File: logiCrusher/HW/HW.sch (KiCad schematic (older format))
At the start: 11 parts, among them J1 Left, J3 Conn_02x05_Odd_Even, J4 Right, U3 R-783.3-0.5

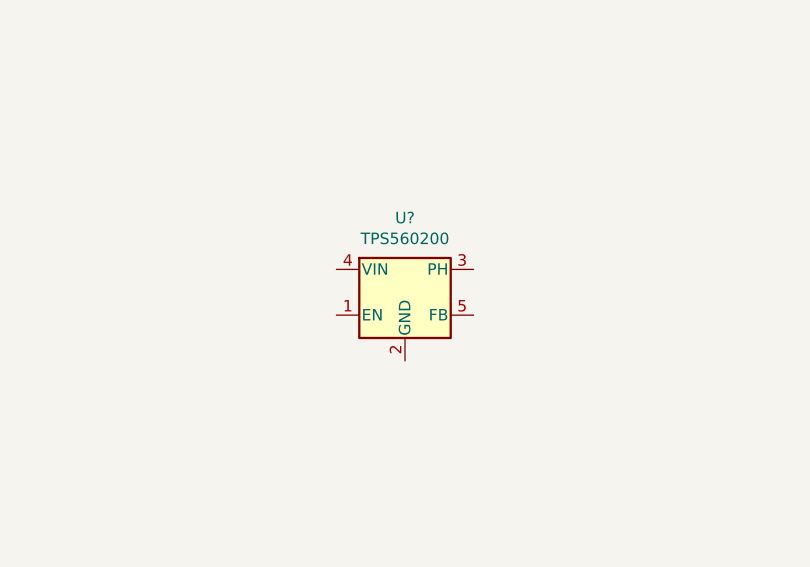
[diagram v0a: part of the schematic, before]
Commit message: Added some deps
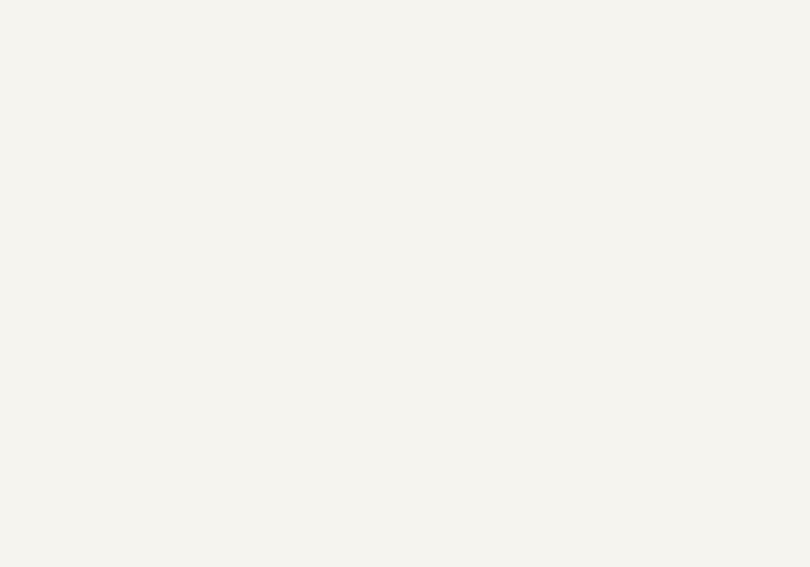
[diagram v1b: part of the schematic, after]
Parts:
- removed U?: TPS560200, Package_TO_SOT_SMD:SOT-23-5, symbol Regulator_Switching:TPS560200
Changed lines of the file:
@@
 Text Label 2900 1950 0    50   ~ 0
 DIN2
-$Comp
-L Regulator_Switching:TPS560200 U?
-U 1 1 5CBCC094
-P 4850 4850
-F 0 "U?" H 4850 5175 50  0000 C CNN
-F 1 "TPS560200" H 4850 5084 50  0000 C CNN
-F 2 "Package_TO_SOT_SMD:SOT-23-5" H 4900 4600 50  0001 L CNN
-F 3 "http://www.ti.com/lit/ds/symlink/tps560200.pdf" H 4600 4500 50  0001 C CNN
-	1    4850 4850
-	1    0    0    -1
-$EndComp
 $EndSCHEMATC
